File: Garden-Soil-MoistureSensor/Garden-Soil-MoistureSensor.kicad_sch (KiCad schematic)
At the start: 10 parts, among them IC1 CD74HC4067M96, IC2 CD74HC4067M96, J1 Conn_01x15, J2 Conn_01x15, U1 1043

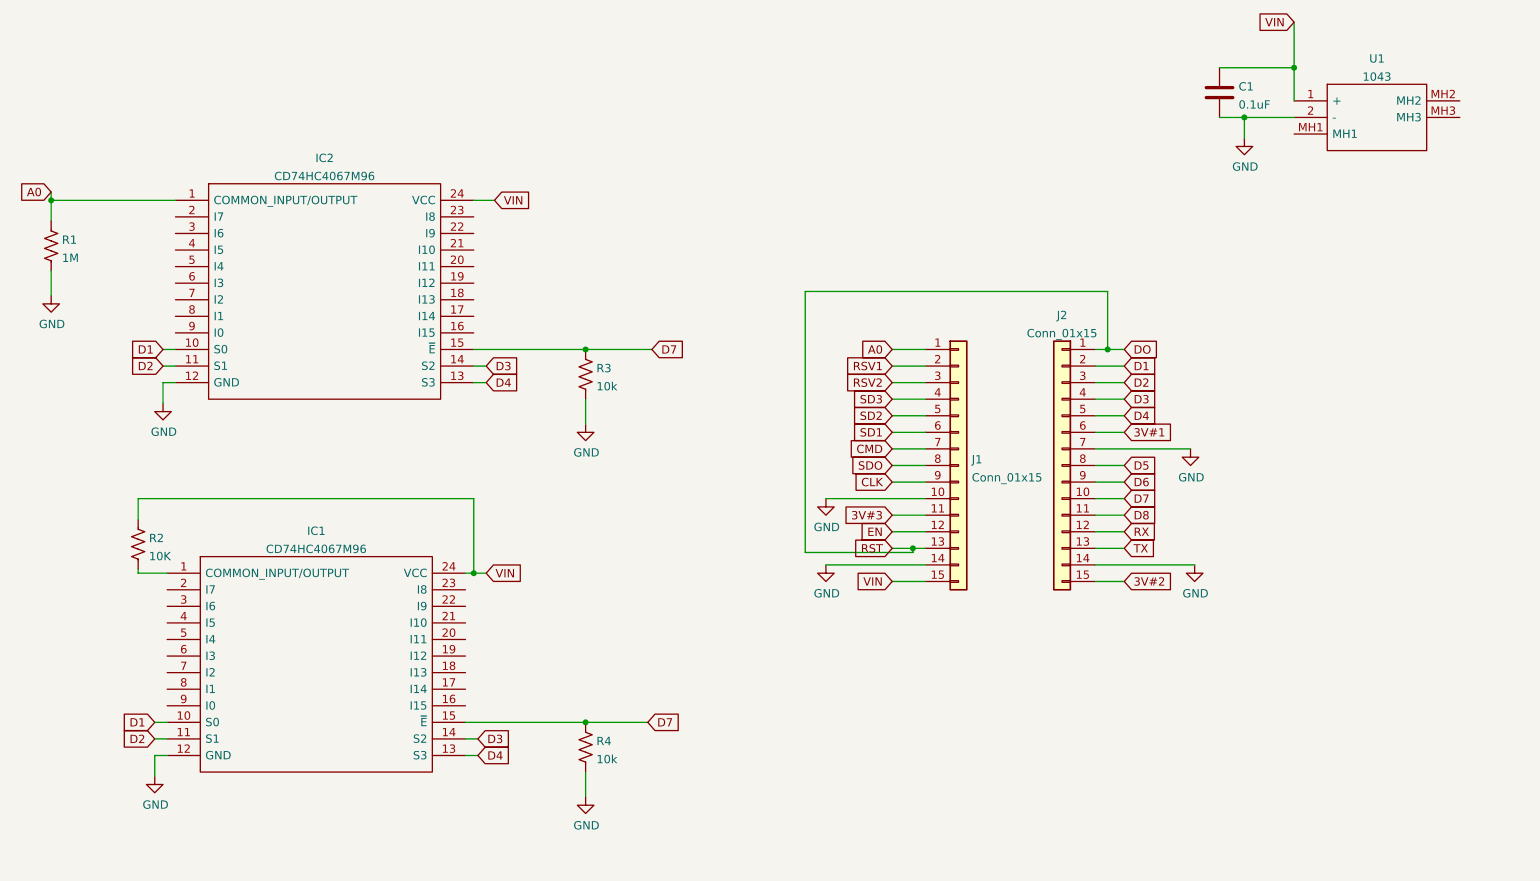
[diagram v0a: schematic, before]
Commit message: got the basics into the schematic. I may rename this model "Liquid Squid" or something like that.
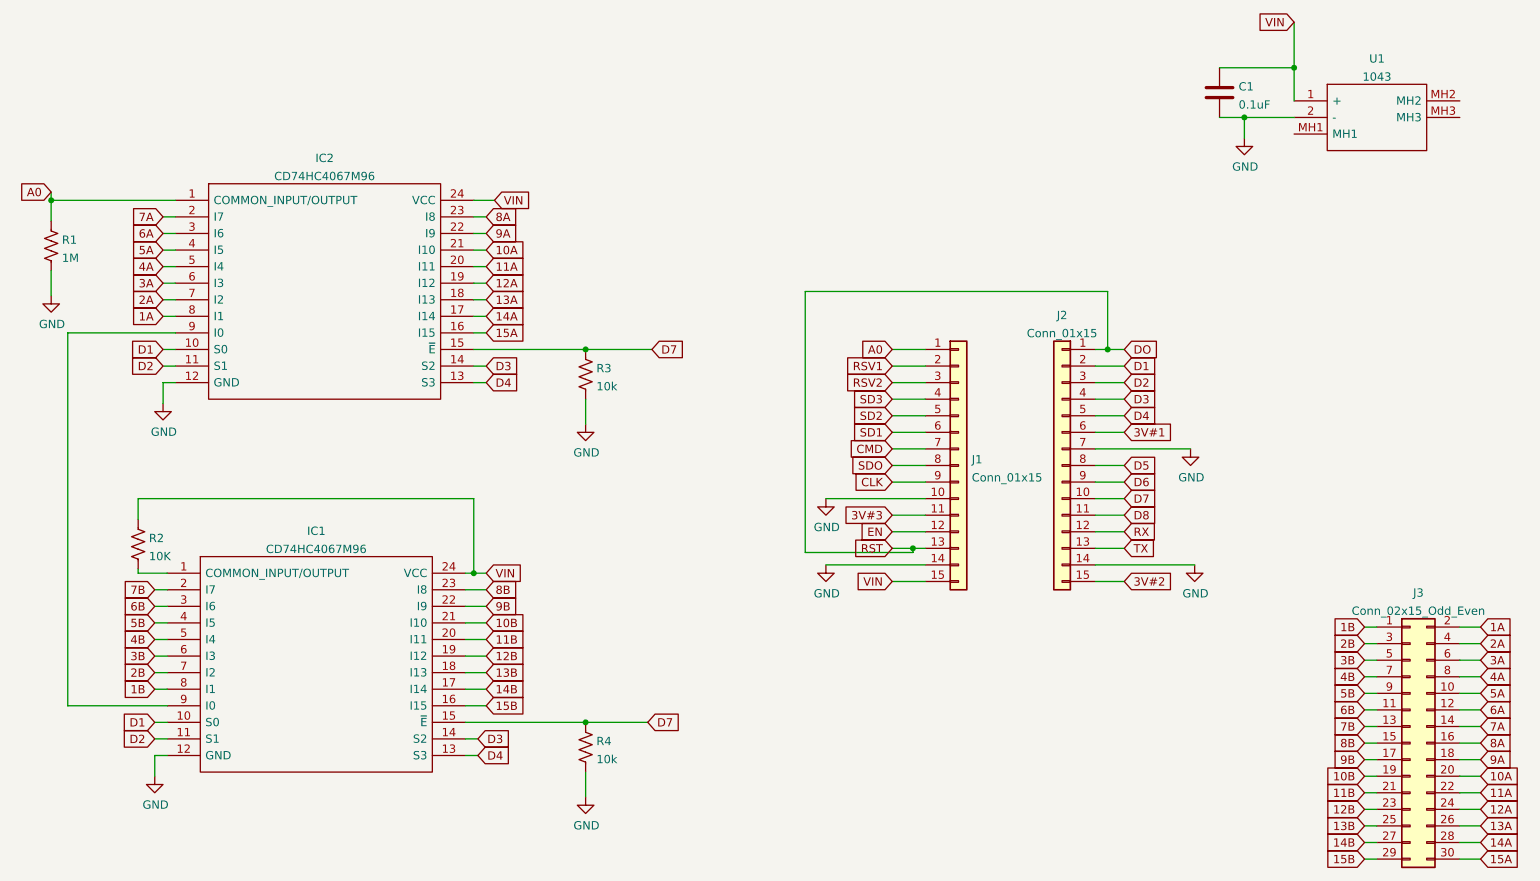
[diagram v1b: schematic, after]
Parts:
- added J3: Conn_02x15_Odd_Even, Connector_PinSocket_2.54mm:PinSocket_2x15_P2.54mm_Horizontal, symbol Connector_Generic:Conn_02x15_Odd_Even
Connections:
- net 15A: now reaches IC2.16 (I15)
- net 15A: now also J3.30 (Pin_30)
- net 14A: now reaches IC2.17 (I14)
- net 14A: now also J3.28 (Pin_28)
- net 13A: now reaches IC2.18 (I13)
- net 13A: now also J3.26 (Pin_26)
- net 12A: now reaches IC2.19 (I12)
- net 12A: now also J3.24 (Pin_24)
- net 7A: now reaches IC2.2 (I7)
- net 7A: now also J3.14 (Pin_14)
- net 11A: now reaches IC2.20 (I11)
- net 11A: now also J3.22 (Pin_22)
- net 10A: now reaches IC2.21 (I10)
- net 10A: now also J3.20 (Pin_20)
- net 9A: now reaches IC2.22 (I9)
- net 9A: now also J3.18 (Pin_18)
- net 8A: now reaches IC2.23 (I8)
- net 8A: now also J3.16 (Pin_16)
- net 6A: now reaches IC2.3 (I6)
- net 6A: now also J3.12 (Pin_12)
- net 5A: now reaches IC2.4 (I5)
- net 5A: now also J3.10 (Pin_10)
- net 4A: now reaches IC2.5 (I4)
- net 4A: now also J3.8 (Pin_8)
- net 3A: now reaches IC2.6 (I3)
- net 3A: now also J3.6 (Pin_6)
- net 2A: now reaches IC2.7 (I2)
- net 2A: now also J3.4 (Pin_4)
- net 1A: now reaches IC2.8 (I1)
- net 1A: now also J3.2 (Pin_2)
- net at IC2.9 (I0): now also IC1.9 (I0)
- net 15B: now reaches IC1.16 (I15)
- net 15B: now also J3.29 (Pin_29)
- net 14B: now reaches IC1.17 (I14)
- net 14B: now also J3.27 (Pin_27)
- net 13B: now reaches IC1.18 (I13)
- net 13B: now also J3.25 (Pin_25)
- net 12B: now reaches IC1.19 (I12)
- net 12B: now also J3.23 (Pin_23)
- net 7B: now reaches IC1.2 (I7)
- net 7B: now also J3.13 (Pin_13)
- net 11B: now reaches IC1.20 (I11)
- net 11B: now also J3.21 (Pin_21)
- net 10B: now reaches IC1.21 (I10)
- net 10B: now also J3.19 (Pin_19)
- net 9B: now reaches IC1.22 (I9)
- net 9B: now also J3.17 (Pin_17)
- net 8B: now reaches IC1.23 (I8)
- net 8B: now also J3.15 (Pin_15)
- net 6B: now reaches IC1.3 (I6)
- net 6B: now also J3.11 (Pin_11)
- net 5B: now reaches IC1.4 (I5)
- net 5B: now also J3.9 (Pin_9)
- net 4B: now reaches IC1.5 (I4)
- net 4B: now also J3.7 (Pin_7)
- net 3B: now reaches IC1.6 (I3)
- net 3B: now also J3.5 (Pin_5)
- net 2B: now reaches IC1.7 (I2)
- net 2B: now also J3.3 (Pin_3)
- net 1B: now reaches IC1.8 (I1)
- net 1B: now also J3.1 (Pin_1)
